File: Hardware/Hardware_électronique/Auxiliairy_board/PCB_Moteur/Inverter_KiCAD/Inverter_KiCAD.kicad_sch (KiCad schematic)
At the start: 61 parts, among them J1 Conn_02x02_Top_Bottom, J2 173010542, J3 Conn_02x05_Odd_Even, J4 Conn_01x02, J5 Conn_01x02, Q1 IRF540N, Q2 IRF540N, Q3 IRF540N, Q4 IRF540N, Q5 SQ2310ES, U1 MIC4606, U2 GO 10-SME/SP3, U3 GO 10-SME/SP3, U4 AZ1117-3.3, U5 MAX3097ECSE+

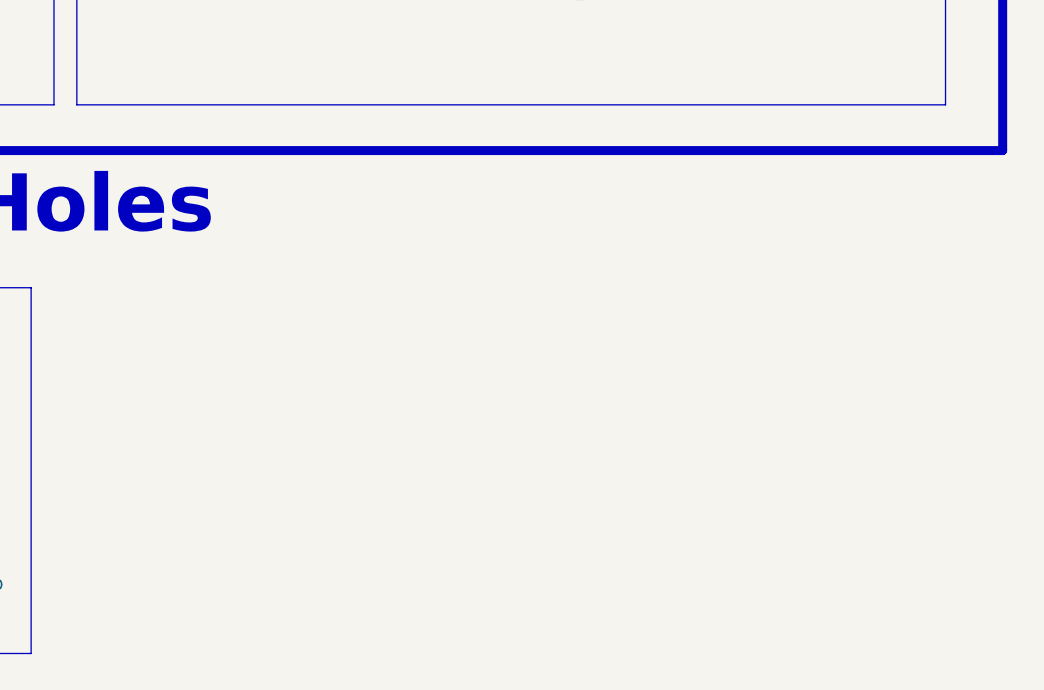
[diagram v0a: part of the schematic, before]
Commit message: Add files via upload
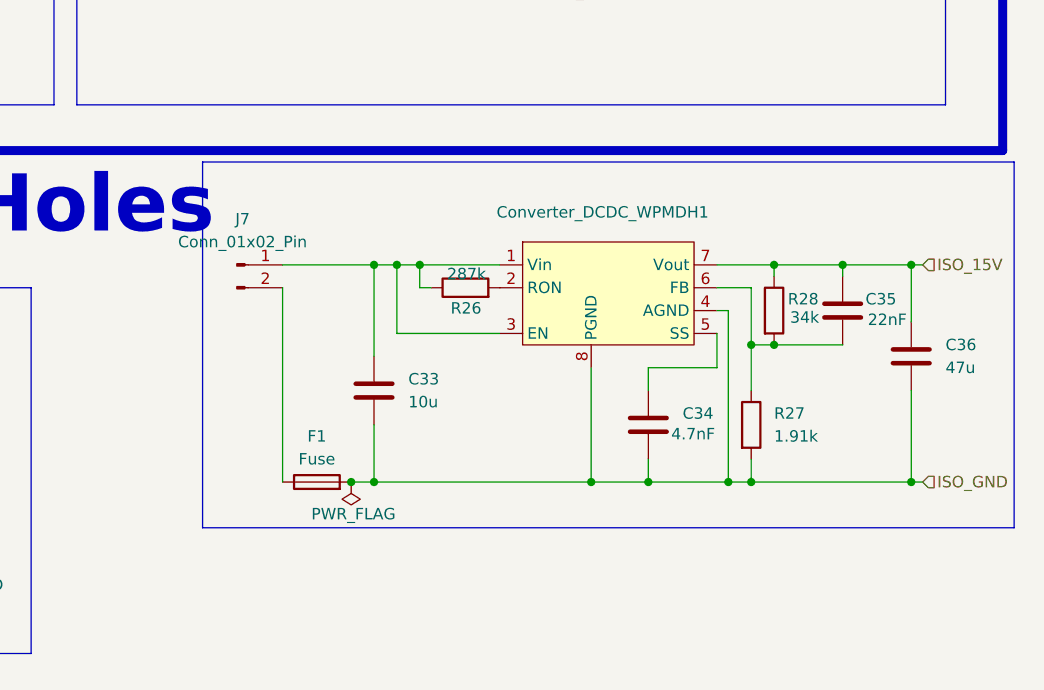
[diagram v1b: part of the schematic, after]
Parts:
- added C33: 10u, symbol Device:C
- added C34: 4.7nF, symbol Device:C
- added C35: 22nF, symbol Device:C
- added C36: 47u, symbol Device:C
- added Converter_DCDC_WPMDH1: ~, Custom:Converter_DCDC, symbol Custom:Converter_DCDC
- added F1: Fuse, Custom:0031.8201, symbol Device:Fuse
- added J7: Conn_01x02_Pin, Connector_AMASS:AMASS_XT60PW-F_1x02_P7.20mm_Horizontal, symbol Connector:Conn_01x02_Pin
- added R26: 287k, symbol Device:R
- added R27: 1.91k, symbol Device:R
- added R28: 34k, symbol Device:R
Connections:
- new net: C34.1, Converter_DCDC_WPMDH1.5 (SS)
- new net: F1.1, J7.2 (Pin_2)
- new net: C35.2, Converter_DCDC_WPMDH1.6 (FB), R27.1, R28.2
- new net: C33.1, Converter_DCDC_WPMDH1.1 (Vin), Converter_DCDC_WPMDH1.3 (EN), J7.1 (Pin_1), R26.1
- new net: Converter_DCDC_WPMDH1.2 (RON), R26.2
- new net ISO_15V: C35.1, C36.1, Converter_DCDC_WPMDH1.7 (Vout), R28.1
- new net ISO_GND: C33.2, C34.2, C36.2, Converter_DCDC_WPMDH1.4 (AGND), Converter_DCDC_WPMDH1.8 (PGND), F1.2, R27.2
